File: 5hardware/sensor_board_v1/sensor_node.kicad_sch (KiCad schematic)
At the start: 31 parts, among them J1 Conn_01x09_Pin, Q2 AO3401A, Q3 AO3400A, SW1 SW_Push, SW2 SW_Push, U12 APDS-9960, U13 SHT31-DIS, U17 BH1750FVI-TR, U3 INA219AxDCN, U4 2N7002DW, U7 XC6206PxxxMR, U8 TPL5110

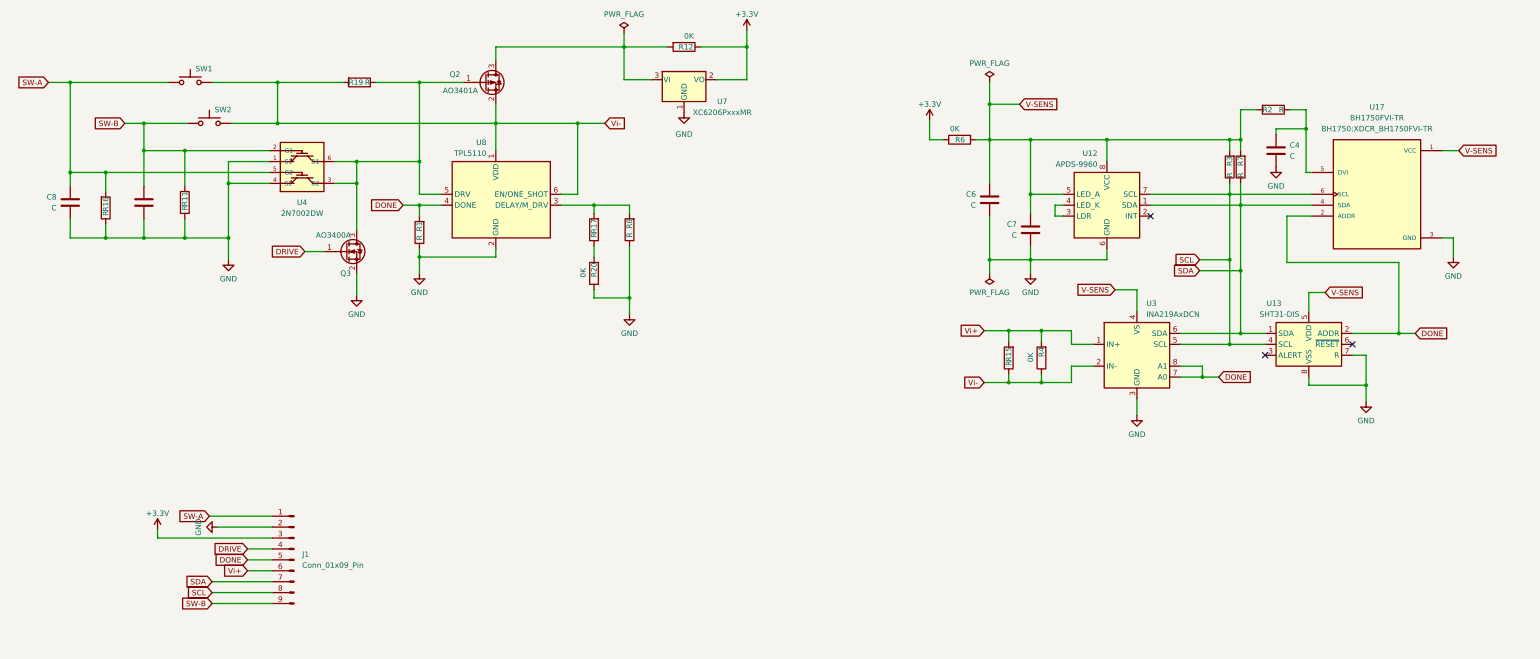
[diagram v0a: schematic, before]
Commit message: update PCBs.
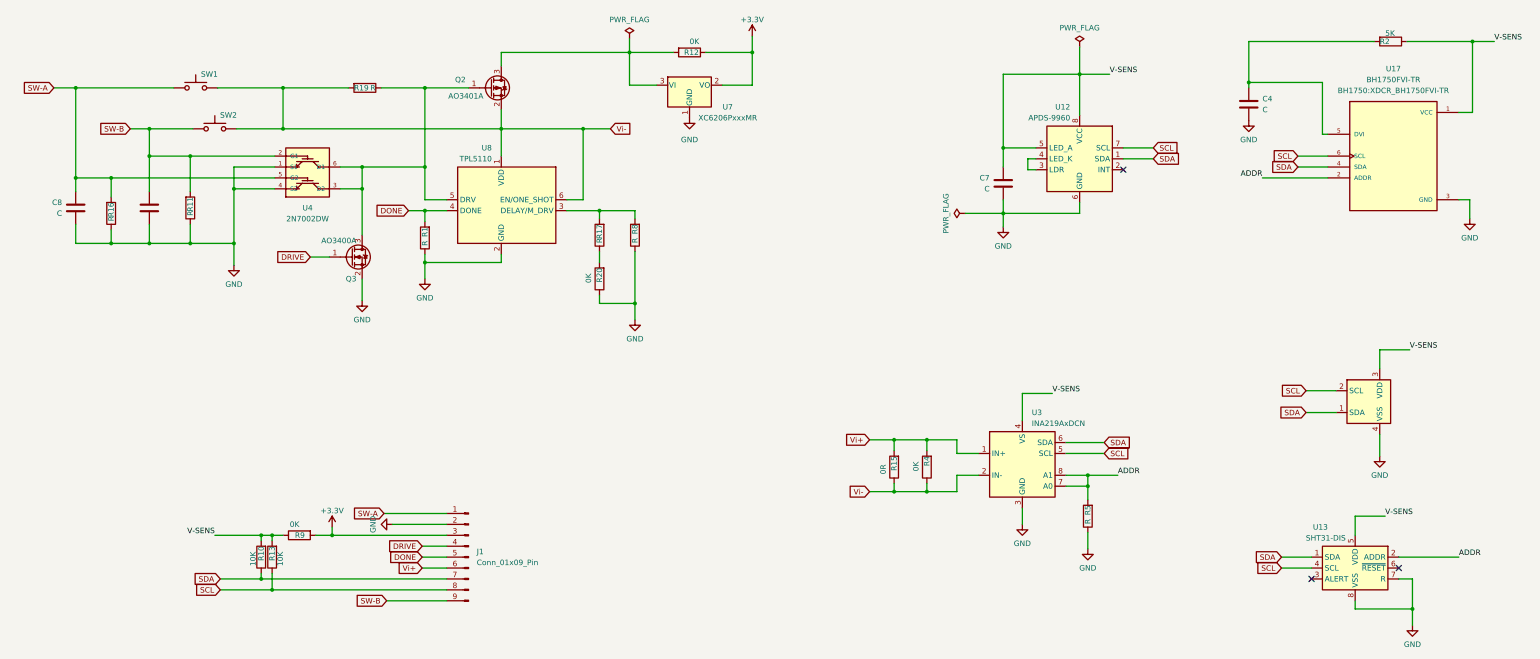
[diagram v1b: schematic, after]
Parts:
- removed C6: C, Capacitor_SMD:C_0603_1608Metric, symbol Device:C
- removed R3, R7: R, Resistor_SMD:R_0603_1608Metric, symbol Device:R
- removed R6: 0K, A_SensorNode:Jumpper, symbol Device:R
- added R10, R13: 10K, Resistor_SMD:R_0603_1608Metric, symbol Device:R
- added R5: R, Resistor_SMD:R_0603_1608Metric, symbol Device:R
- added R9: 0K, A_SensorNode:Jumpper, symbol Device:R
- added U1: SHT4x, Sensor_Humidity:Sensirion_DFN-4_1.5x1.5mm_P0.8mm_SHT4x_NoCentralPad, symbol Sensor_Humidity:SHT4x
- R15: value R -> 0R
- R2: value R -> 5K
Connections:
- net +3.3V: now also R9.2
- net DONE: no longer U13.2 (ADDR), U17.2 (ADDR), U3.7 (A0), U3.8 (A1)
- net GND: now also R5.1, U1.4 (VSS)
- net SCL: now also R13.1, U1.2 (SCL)
- net SDA: now also R10.1, U1.1 (SDA)
- net V-SENS: now also R2.1, R10.2, R13.2, R9.1, U1.3 (VDD); no longer R2.2
- net at C4.1, U17.5 (DVI): now also R2.2; no longer R2.1
- new net ADDR: R5.2, U13.2 (ADDR), U17.2 (ADDR), U3.7 (A0), U3.8 (A1)
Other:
- moved on the sheet: C4, C7, C8, J1, Q2, Q3, R1, R11, R12, R15, R16, R17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
